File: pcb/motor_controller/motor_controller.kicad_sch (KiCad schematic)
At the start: 5 parts, among them U1 STM32F446RETx, U2 DRV8323RHRGZT, U3 LDFM33PUR, U4 MA702GQ-Z, U5 MCP2542FDT-H/MNY

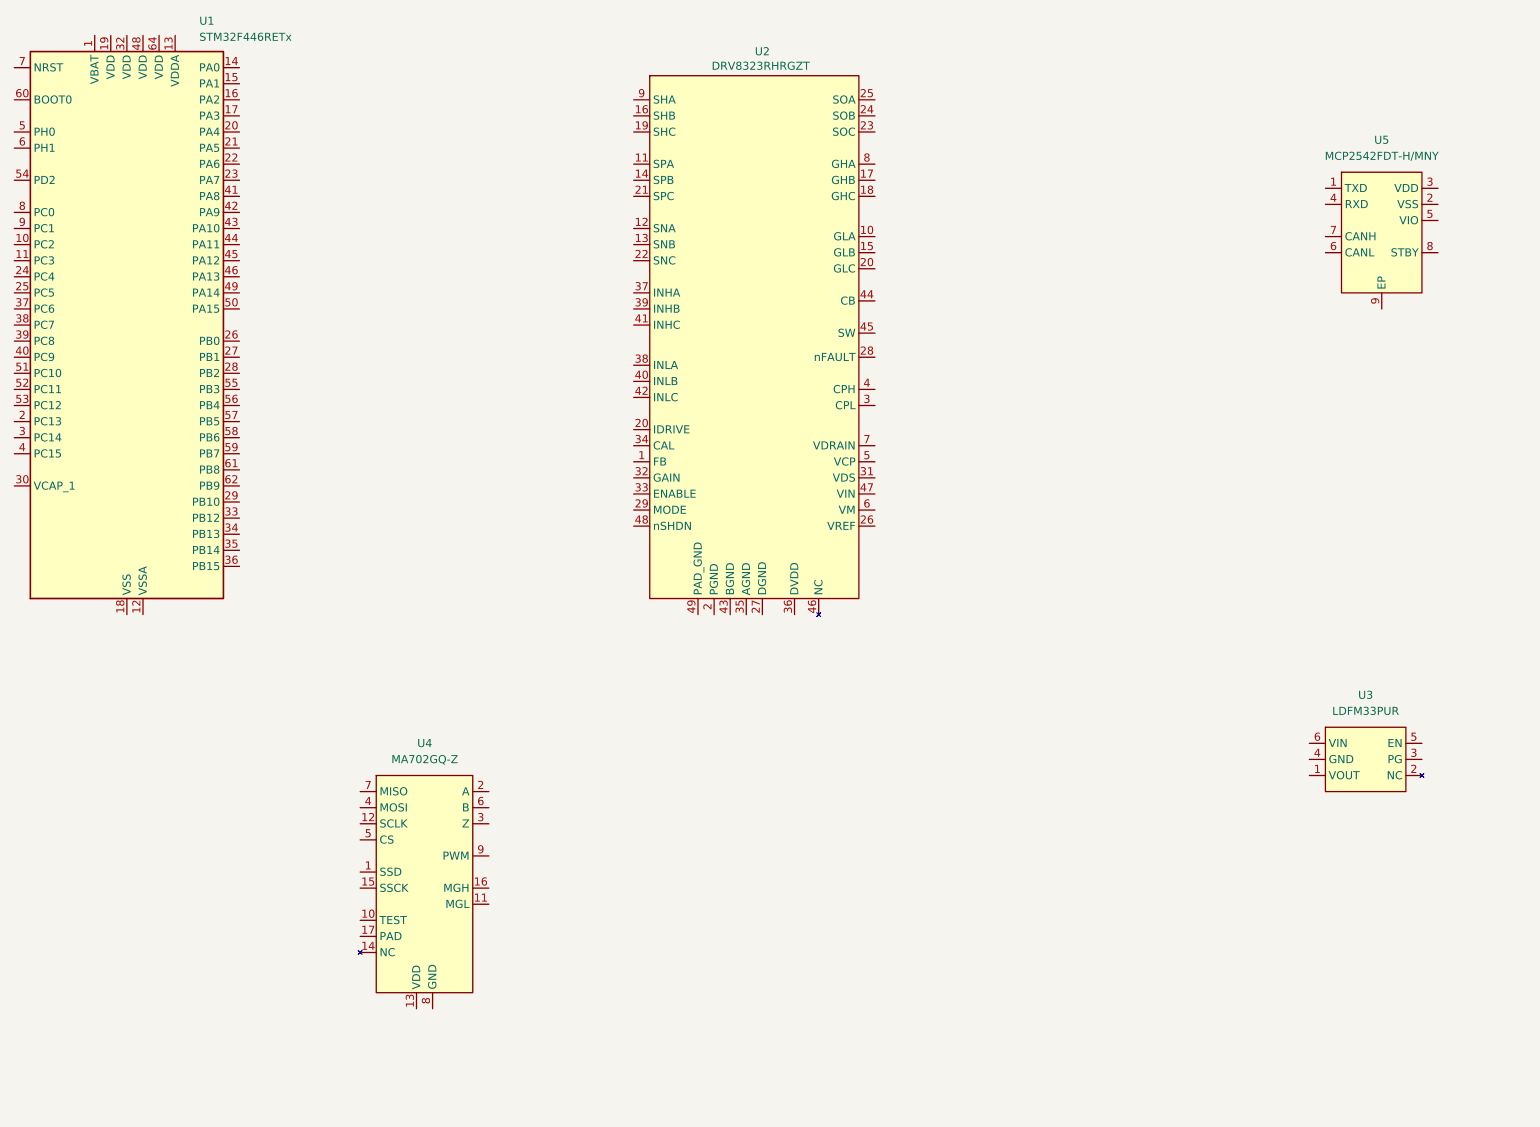
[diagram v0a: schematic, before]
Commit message: Latest update.
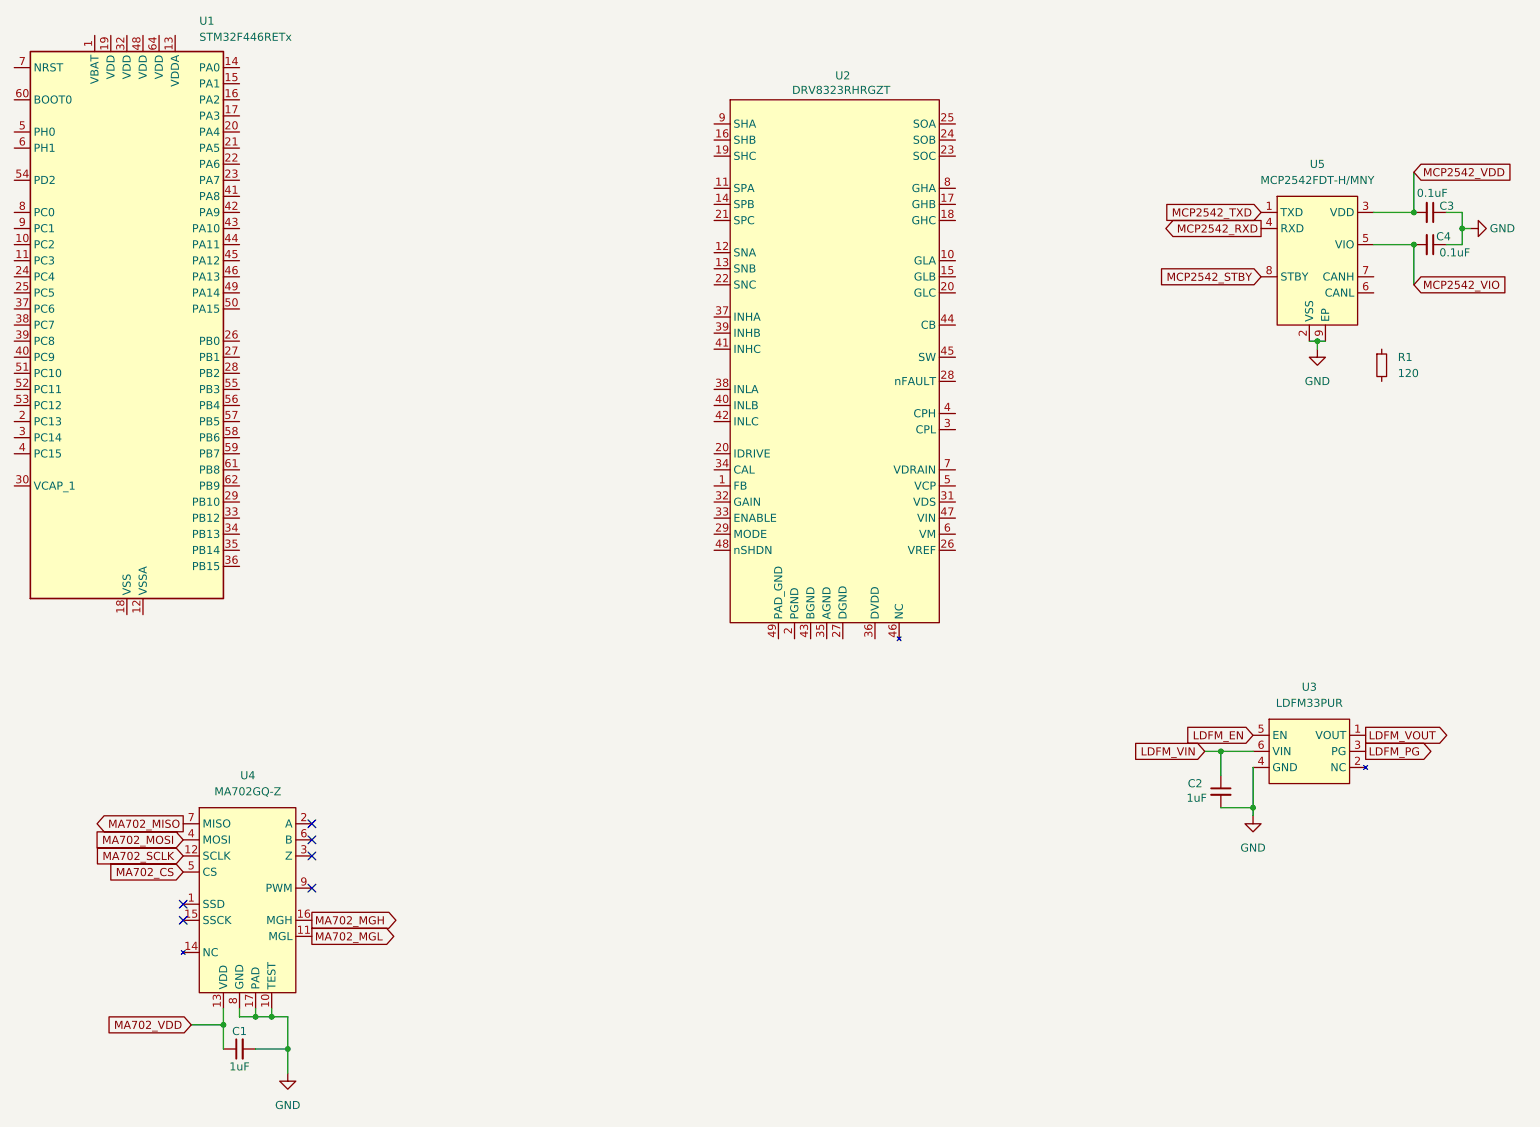
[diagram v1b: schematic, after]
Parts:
- added C1, C2: 1uF, symbol Device:C_Small
- added C3, C4: 0.1uF, symbol Device:C_Small
- added R1: 120, symbol Device:R_Small
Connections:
- net GND: now reaches U4.10 (TEST)
- net GND: now also U3.4 (GND), U4.17 (PAD), U4.8 (GND), U5.2 (VSS), U5.9 (EP), C1.2, C2.2, C3.1, C4.1
- net MA702_MGL: now reaches U4.11 (MGL)
- net MA702_SCLK: now reaches U4.12 (SCLK)
- net MA702_VDD: now reaches U4.13 (VDD)
- net MA702_VDD: now also C1.1
- net MA702_MGH: now reaches U4.16 (MGH)
- net MA702_MOSI: now reaches U4.4 (MOSI)
- net MA702_CS: now reaches U4.5 (CS)
- net MA702_MISO: now reaches U4.7 (MISO)
- net MCP2542_TXD: now reaches U5.1 (TXD)
- net MCP2542_VDD: now reaches U5.3 (VDD)
- net MCP2542_VDD: now also C3.2
- net MCP2542_RXD: now reaches U5.4 (RXD)
- net MCP2542_VIO: now reaches U5.5 (VIO)
- net MCP2542_VIO: now also C4.2
- net MCP2542_STBY: now reaches U5.8 (STBY)
- net LDFM_VOUT: now reaches U3.1 (VOUT)
- net LDFM_PG: now reaches U3.3 (PG)
- net LDFM_EN: now reaches U3.5 (EN)
- net LDFM_VIN: now reaches U3.6 (VIN)
- net LDFM_VIN: now also C2.1
- no-connect marks 0 -> 6
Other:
- moved on the sheet: U2, U3, U4, U5
